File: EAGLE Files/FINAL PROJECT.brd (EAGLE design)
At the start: 105.4 x 49.5 mm, 18 parts, among them J1 BATTERY, U1 9_to_3.3_VREG

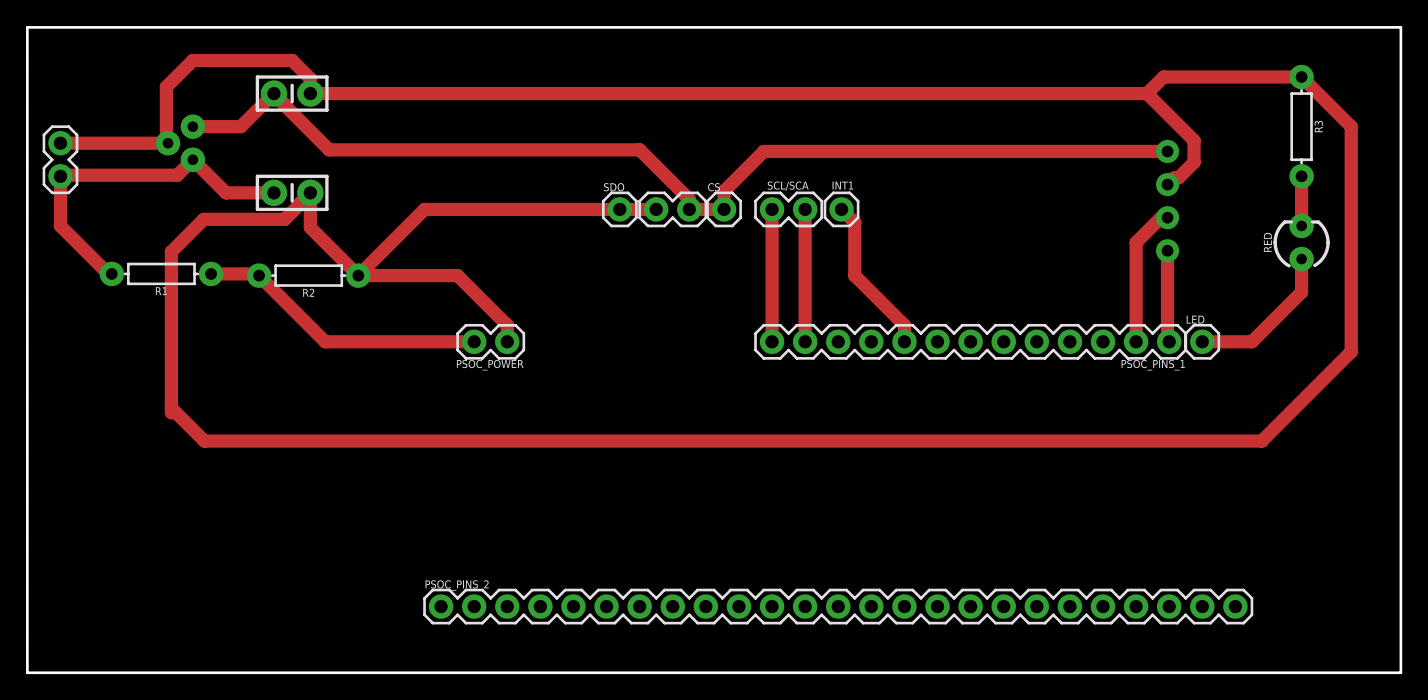
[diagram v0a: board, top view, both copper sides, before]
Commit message: final EAGLE files
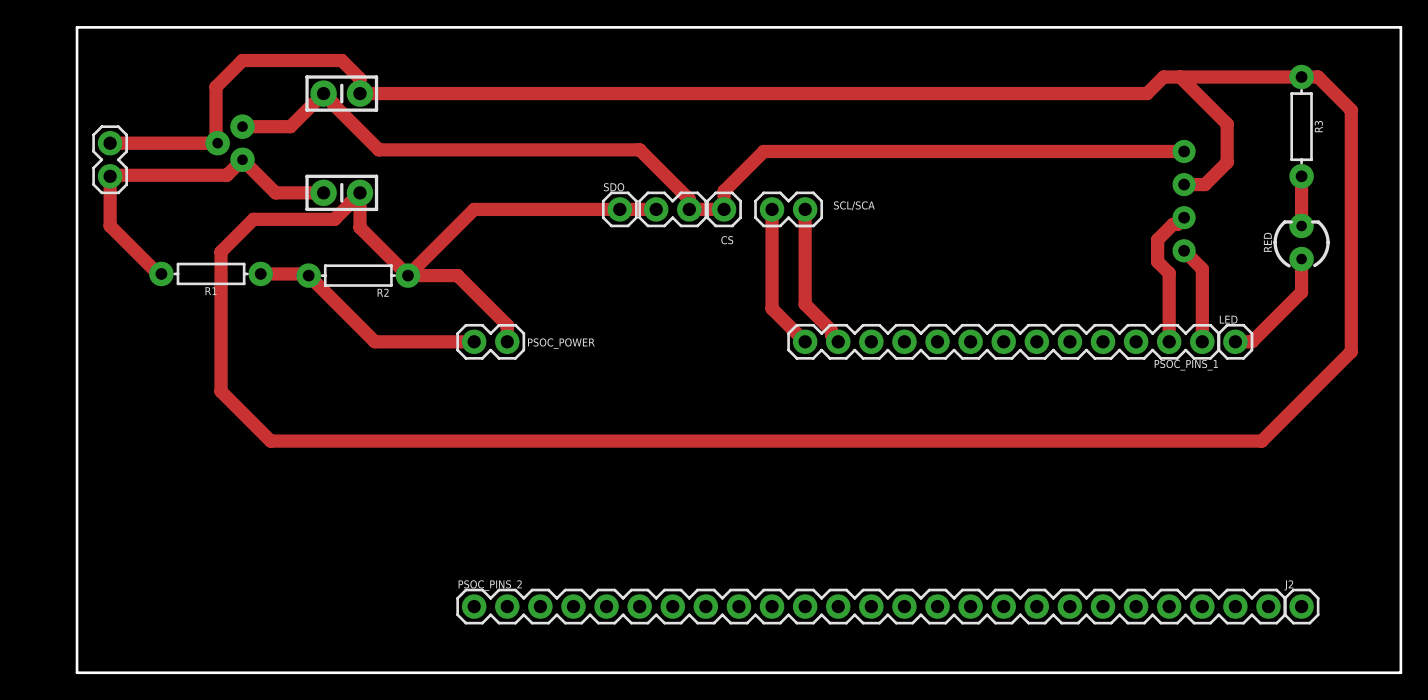
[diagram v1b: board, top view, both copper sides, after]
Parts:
- removed INT1: (no value), SparkFun-Connectors:1X01
- added J2: (no value), SparkFun-Connectors:1X01
- moved U1 3.81 mm to (16.5, 40.6)
- moved J1 3.81 mm to (6.35, 40.6)
- moved C3 3.81 mm to (24.1, 44.5)
- moved C4 3.81 mm to (24.1, 36.8)
- moved R1 3.81 mm to (14.1, 30.6)
- moved R2 3.81 mm to (25.4, 30.5)
- moved PSOC_PINS_1 2.54 mm to (90.2, 25.4)
- moved PSOC_PINS_2 2.54 mm to (34.3, 5.08)
- moved LED 2.54 mm to (92.7, 25.4)
- moved HC-05 1.27 mm to (105.3, 36.2)
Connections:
- removed net INT1: INT1.1, PSOC_PINS_1.9
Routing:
- net GND: track 301.8 -> 288.7 mm
- net INT1: track 12.2 -> 0.00 mm
- net 5V: track 22.3 -> 18.5 mm
- net VDD: track 82.7 -> 80.2 mm
- net LED: track 11.7 -> 9.20 mm
- net SCL: track 10.2 -> 11.2 mm
- net SCA: track 10.2 -> 11.2 mm
- net RX: track 7.04 -> 7.56 mm
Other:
- board size 105.4 x 49.5 mm -> 101.6 x 49.5 mm
